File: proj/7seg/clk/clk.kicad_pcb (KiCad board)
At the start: 2 copper layers, 50 x 15 mm, 27 parts, among them J1 Conn_01x02_Pin, J2 USB_A, J3 USB_C_Receptacle_PowerOnly_6P, SW1 SW_Push, SW2 SW_Push, U1 LTC-4627JG, U2 74HC595, U3 74HC595, U4 ATtiny402-SS

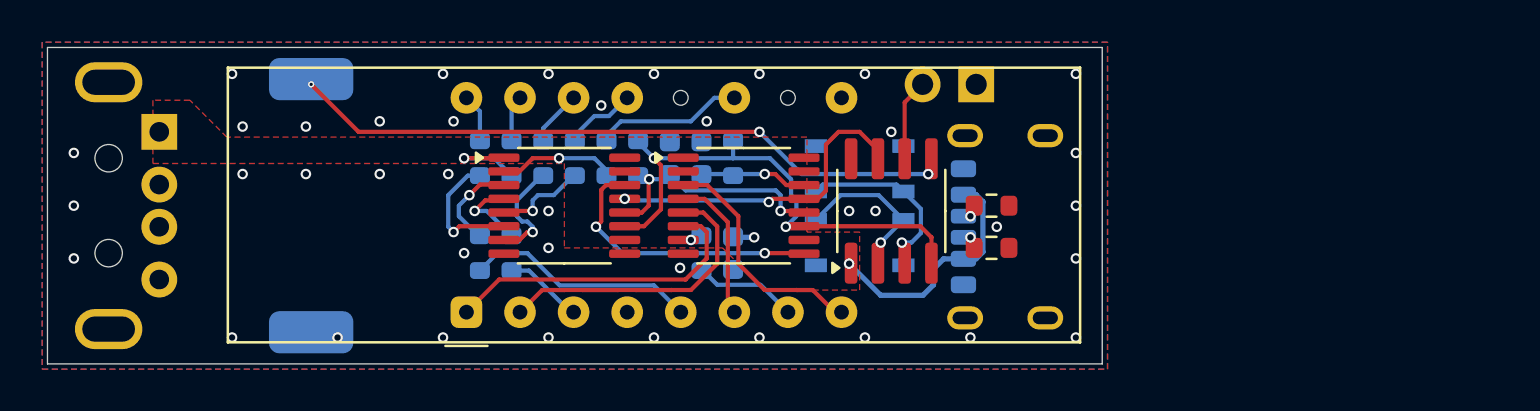
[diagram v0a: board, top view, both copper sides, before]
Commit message: -
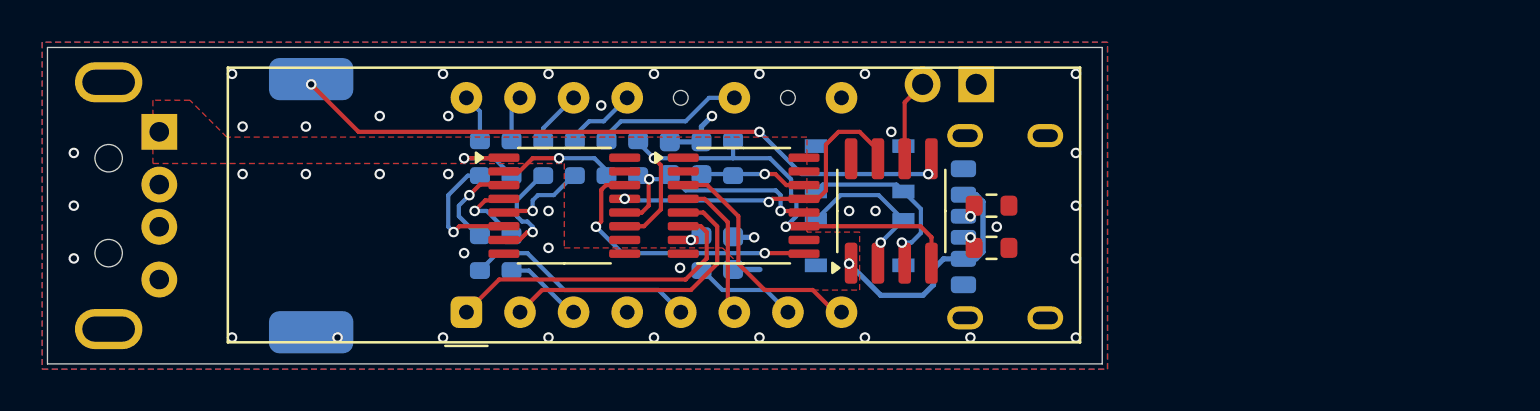
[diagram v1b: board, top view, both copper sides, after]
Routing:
- net GND: track 0.00 -> 4.21 mm
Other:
- board text added: "AVR CLK"
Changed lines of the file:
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@@
 		(layer "Edge.Cuts")
+	)
+	(gr_text "AVR CLK"
+		(at 78.75 102.25 90)
+		(layer "F.Mask")
+		(effects
+			(font
+				(size 1 1)
+				(thickness 0.2)
+				(bold yes)
+			)
+		)
 	)
 	(gr_text "C"
@@
 	)
 	(via
-		(at 90.5 96)
+		(at 90.25 95.75)
 		(size 0.5)
 		(drill 0.3)
@@
 	)
 	(via
-		(at 87 96)
+		(at 87 95.75)
 		(size 0.5)
 		(drill 0.3)
@@
 	)
 	(via
-		(at 102.5 96)
+		(at 102.75 95.75)
 		(size 0.5)
 		(drill 0.3)
@@
 		(layers "F.Cu" "B.Cu")
 		(free yes)
+		(net 2)
+	)
+	(segment
+		(start 100.75 96.975)
+		(end 102.25 96.975)
+		(width 0.25)
+		(layer "B.Cu")
+		(net 2)
+	)
+	(segment
+		(start 102.25 96.975)
+		(end 102.25 96.25)
+		(width 0.25)
+		(layer "B.Cu")
+		(net 2)
+	)
+	(segment
+		(start 103.75 103.025)
+		(end 105.025 103.025)
+		(width 0.25)
+		(layer "B.Cu")
+		(net 2)
+	)
+	(segment
+		(start 102.25 96.25)
+		(end 102.75 95.75)
+		(width 0.25)
+		(layer "B.Cu")
 		(net 2)
 	)
@@
 	(via
 		(at 83.75 94.25)
-		(size 0.3)
-		(drill 0.15)
+		(size 0.5)
+		(drill 0.3)
 		(layers "F.Cu" "B.Cu")
 		(net 9)
@@
 	)
 	(segment
-		(start 97.8675 95.75)
-		(end 98.73 94.8875)
-		(width 0.2)
-		(layer "B.Cu")
-		(net 14)
-	)
-	(segment
-		(start 96.25 96.675)
-		(end 97.175 95.75)
-		(width 0.2)
-		(layer "B.Cu")
-		(net 14)
-	)
-	(segment
 		(start 96.25 96.925)
 		(end 96.25 96.675)
@@
 	)
 	(segment
-		(start 97.175 95.75)
-		(end 97.8675 95.75)
+		(start 96.925 96)
+		(end 97.6175 96)
+		(width 0.2)
+		(layer "B.Cu")
+		(net 14)
+	)
+	(segment
+		(start 97.6175 96)
+		(end 98.73 94.8875)
+		(width 0.2)
+		(layer "B.Cu")
+		(net 14)
+	)
+	(segment
+		(start 96.25 96.675)
+		(end 96.925 96)
 		(width 0.2)
 		(layer "B.Cu")
@@
 	)
 	(segment
-		(start 91.75 103.075)
+		(start 100.219 103.9965)
+		(end 95.7465 103.9965)
+		(width 0.2)
+		(layer "B.Cu")
+		(net 18)
+	)
+	(segment
+		(start 101.27 105.0475)
+		(end 100.219 103.9965)
+		(width 0.2)
+		(layer "B.Cu")
+		(net 18)
+	)
+	(segment
+		(start 94 102.25)
 		(end 92.575 102.25)
 		(width 0.2)
@@
 	)
 	(segment
-		(start 95.526 103.776)
-		(end 99.9985 103.776)
+		(start 95.7465 103.9965)
+		(end 94 102.25)
 		(width 0.2)
 		(layer "B.Cu")
@@
 	)
 	(segment
-		(start 99.9985 103.776)
-		(end 101.27 105.0475)
-		(width 0.2)
-		(layer "B.Cu")
-		(net 18)
-	)
-	(segment
-		(start 94 102.25)
-		(end 95.526 103.776)
-		(width 0.2)
-		(layer "B.Cu")
-		(net 18)
-	)
-	(segment
 		(start 92.575 102.25)
-		(end 94 102.25)
+		(end 91.75 103.075)
 		(width 0.2)
 		(layer "B.Cu")
@@
 	)
 	(segment
+		(start 102.6125 94.8875)
+		(end 101.5 96)
+		(width 0.2)
+		(layer "B.Cu")
+		(net 20)
+	)
+	(segment
 		(start 103.81 94.8875)
-		(end 102.8625 94.8875)
+		(end 102.6125 94.8875)
 		(width 0.2)
 		(layer "B.Cu")
@@
 	)
 	(segment
-		(start 102.8625 94.8875)
-		(end 101.75 96)
-		(width 0.2)
-		(layer "B.Cu")
-		(net 20)
-	)
-	(segment
-		(start 101.75 96)
-		(end 98.429251 96)
+		(start 98.429251 96)
+		(end 97.75 96.679251)
 		(width 0.2)
 		(layer "B.Cu")
@@
 	)
 	(segment
-		(start 98.429251 96)
-		(end 97.75 96.679251)
+		(start 101.5 96)
+		(end 98.429251 96)
 		(width 0.2)
 		(layer "B.Cu")
@@
 	)
 	(segment
-		(start 105.0525 103.75)
-		(end 106.35 105.0475)
-		(width 0.2)
-		(layer "B.Cu")
-		(net 24)
-	)
-	(segment
-		(start 102.325 103.075)
-		(end 103 103.75)
-		(width 0.2)
-		(layer "B.Cu")
-		(net 24)
-	)
-	(segment
-		(start 103 103.75)
-		(end 105.0525 103.75)
-		(width 0.2)
-		(layer "B.Cu")
-		(net 24)
-	)
-	(segment
 		(start 102.25 103.075)
 		(end 102.325 103.075)
@@
 		(net 24)
 	)
+	(segment
+		(start 102.325 103.075)
+		(end 103.2465 103.9965)
+		(width 0.2)
+		(layer "B.Cu")
+		(net 24)
+	)
+	(segment
+		(start 103.2465 103.9965)
+		(end 105.299 103.9965)
+		(width 0.2)
+		(layer "B.Cu")
+		(net 24)
+	)
+	(segment
+		(start 105.299 103.9965)
+		(end 106.35 105.0475)
+		(width 0.2)
+		(layer "B.Cu")
+		(net 24)
+	)
 	(via
 		(at 101.75 101.625)
@@
 	)
 	(segment
-		(start 106.788839 104)
-		(end 107.53013 104)
-		(width 0.2)
-		(layer "F.Cu")
-		(net 32)
-	)
-	(segment
 		(start 102.525 99.025)
 		(end 104 100.5)
@@
 	)
 	(segment
+		(start 101.3875 99.025)
+		(end 102.525 99.025)
+		(width 0.2)
+		(layer "F.Cu")
+		(net 32)
+	)
+	(segment
+		(start 108.57763 105.0475)
+		(end 108.89 105.0475)
+		(width 0.2)
+		(layer "F.Cu")
+		(net 32)
+	)
+	(segment
 		(start 104 102.75)
 		(end 105.2465 103.9965)
@@
 	)
 	(segment
-		(start 106.785339 103.9965)
-		(end 106.788839 104)
-		(width 0.2)
-		(layer "F.Cu")
-		(net 32)
-	)
-	(segment
-		(start 105.2465 103.9965)
-		(end 106.785339 103.9965)
-		(width 0.2)
-		(layer "F.Cu")
-		(net 32)
-	)
-	(segment
-		(start 108.57763 105.0475)
-		(end 108.89 105.0475)
-		(width 0.2)
-		(layer "F.Cu")
-		(net 32)
-	)
-	(segment
-		(start 101.3875 99.025)
-		(end 102.525 99.025)
-		(width 0.2)
-		(layer "F.Cu")
-		(net 32)
-	)
-	(segment
-		(start 107.53013 104)
+		(start 107.52663 103.9965)
 		(end 108.57763 105.0475)
 		(width 0.2)
@@
 	)
 	(segment
+		(start 105.2465 103.9965)
+		(end 107.52663 103.9965)
+		(width 0.2)
+		(layer "F.Cu")
+		(net 32)
+	)
+	(segment
 		(start 102.225 100.975)
 		(end 102.5 101.25)
@@
 	)
 	(segment
-		(start 94.6975 104)
-		(end 93.65 105.0475)
+		(start 101.3875 100.325)
+		(end 102.341426 100.325)
+		(width 0.2)
+		(layer "F.Cu")
+		(net 34)
+	)
+	(segment
+		(start 101.7535 103.9965)
+		(end 94.701 103.9965)
+		(width 0.2)
+		(layer "F.Cu")
+		(net 34)
+	)
+	(segment
+		(start 102.341426 100.325)
+		(end 103 100.983574)
 		(width 0.2)
 		(layer "F.Cu")
@@
 	)
 	(segment
-		(start 95.754661 103.9965)
-		(end 95.751161 104)
-		(width 0.2)
-		(layer "F.Cu")
-		(net 34)
-	)
-	(segment
-		(start 98.291161 104)
-		(end 96.628839 104)
-		(width 0.2)
-		(layer "F.Cu")
-		(net 34)
-	)
-	(segment
-		(start 99.168839 104)
-		(end 99.165339 103.9965)
-		(width 0.2)
-		(layer "F.Cu")
-		(net 34)
-	)
-	(segment
-		(start 95.751161 104)
-		(end 94.6975 104)
-		(width 0.2)
-		(layer "F.Cu")
-		(net 34)
-	)
-	(segment
-		(start 102.341426 100.325)
-		(end 103 100.983574)
-		(width 0.2)
-		(layer "F.Cu")
-		(net 34)
-	)
-	(segment
-		(start 96.625339 103.9965)
-		(end 95.754661 103.9965)
-		(width 0.2)
-		(layer "F.Cu")
-		(net 34)
-	)
-	(segment
-		(start 99.165339 103.9965)
-		(end 98.294661 103.9965)
-		(width 0.2)
-		(layer "F.Cu")
-		(net 34)
-	)
-	(segment
-		(start 98.294661 103.9965)
-		(end 98.291161 104)
-		(width 0.2)
-		(layer "F.Cu")
-		(net 34)
-	)
-	(segment
-		(start 100.831161 104)
-		(end 99.168839 104)
-		(width 0.2)
-		(layer "F.Cu")
-		(net 34)
-	)
-	(segment
-		(start 100.834661 103.9965)
-		(end 100.831161 104)
-		(width 0.2)
-		(layer "F.Cu")
-		(net 34)
-	)
-	(segment
-		(start 101.7535 103.9965)
-		(end 100.834661 103.9965)
+		(start 94.701 103.9965)
+		(end 93.65 105.0475)
 		(width 0.2)
 		(layer "F.Cu")
@@
 		(width 0.2)
 		(layer "F.Cu")
-		(net 34)
-	)
-	(segment
-		(start 101.3875 100.325)
-		(end 102.341426 100.325)
-		(width 0.2)
-		(layer "F.Cu")
-		(net 34)
-	)
-	(segment
-		(start 96.628839 104)
-		(end 96.625339 103.9965)
-		(width 0.2)
-		(layer "F.Cu")

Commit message: -
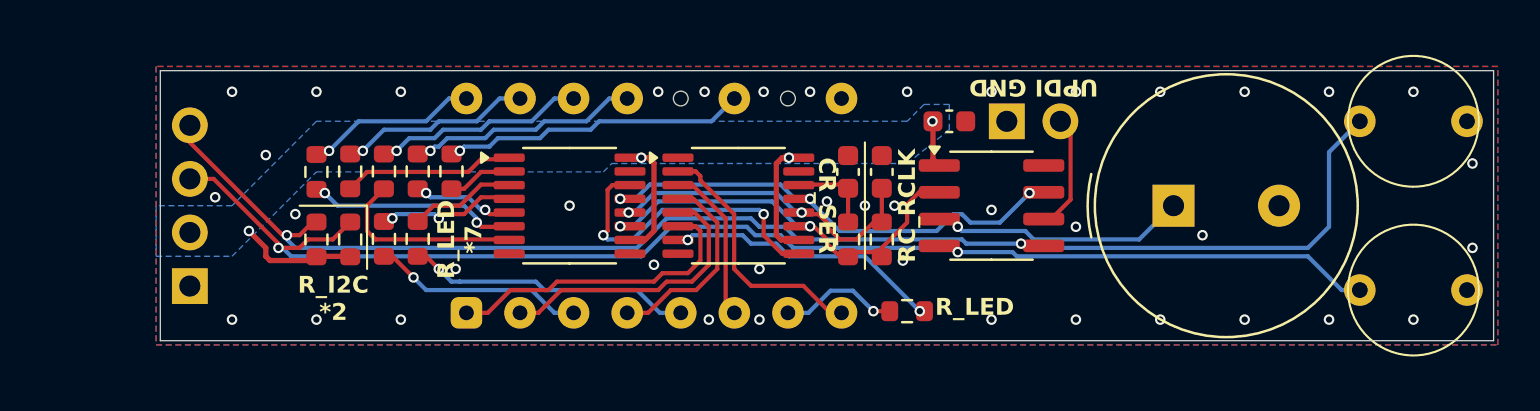
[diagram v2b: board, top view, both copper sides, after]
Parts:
- removed J3: USB_C_Receptacle_PowerOnly_6P, Connector_USB:USB_C_Receptacle_GCT_USB4125-xx-x_6P_TopMnt_Horizontal
- removed LS1: Speaker, Library:PKLCS1212E4001-R1
- added BZ1: Buzzer, Buzzer_Beeper:Buzzer_TDK_PS1240P02BT_D12.2mm_H6.5mm, F.Cu at (124.6, 100.0)
- ?: moved to B.Cu
- C1: value C_Small -> C_RCLK; moved to F.Cu
- C2: value C_Small -> C_SER; moved to F.Cu
- C3, R1, R2, R3, R4, R5, R6, R7, R8: moved to F.Cu
- J2: value USB_A -> Conn_01x04_Pin; footprint Library:USB_A_PLUG_USB-4AM103AS -> Connector_PinHeader_2.54mm:PinHeader_1x04_P2.54mm_Vertical; moved to B.Cu
- R10: value R_Small -> R_SER; moved to F.Cu
- R11, R12: value 5k1 -> R_I2C
- R9: value R_Small -> R_RCLK; moved to F.Cu
- SW1, SW2: footprint Library:alps-skrp -> Library:alps-skrg; moved to F.Cu
- moved ? 52.0 mm to (136.0, 100.0), turned to -90 degrees
- moved G*** 43.4 mm to (127.0, 97.0), turned to -90 degrees
- moved R12 32.0 mm to (84.0, 101.6), turned to 90 degrees
- moved R11 30.4 mm to (85.6, 101.6), turned to 90 degrees
- moved SW1 26.3 mm to (136.0, 104.0)
- moved SW2 26.3 mm to (136.0, 96.0), turned to 0 degrees
- moved R9 12.2 mm to (110.8, 101.6), turned to 90 degrees
- moved C3 12.0 mm to (114.0, 96.0), turned to 0 degrees
- moved R8 10.1 mm to (112.0, 105.0), turned to 180 degrees
- moved C1 10.1 mm to (110.8, 98.4)
- moved R2 7.78 mm to (84.0, 98.4)
- moved J2 7.75 mm to (78.0, 103.8), turned to 0 degrees
- moved R7 7.68 mm to (85.6, 98.4)
- moved R1 7.58 mm to (87.2, 98.4)
- moved R3 7.48 mm to (88.8, 98.4)
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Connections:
- J2 pad 1: VCC -> GND
- J2 pad 2: unconnected-(J2-D--Pad2) -> VCC
- J2 pad 3: unconnected-(J2-D+-Pad3) -> PA1
- J2 pad 4: GND -> PA2
- R1 pad 1: /_SEG0 -> /_SEG1
- R1 pad 2: SEG0 -> SEG1
- R11 pad 1: Net-(J3-CC1) -> VCC
- R11 pad 2: GND -> PA1
- R12 pad 1: Net-(J3-CC2) -> VCC
- R12 pad 2: GND -> PA2
- R2 pad 1: /_SEG1 -> /_SEG2
- R2 pad 2: SEG1 -> SEG2
- R3 pad 1: /_SEG2 -> /_SEG3
- R3 pad 2: SEG2 -> SEG3
- R4 pad 1: /_SEG3 -> /_SEG4
- R4 pad 2: SEG3 -> SEG4
- R5 pad 1: /_SEG4 -> /_SEG5
- R5 pad 2: SEG4 -> SEG5
- R6 pad 1: /_SEG5 -> /_SEG6
- R6 pad 2: SEG5 -> SEG6
- R7 pad 1: /_SEG6 -> /_SEG7
- R7 pad 2: SEG6 -> SEG7
- R8 pad 1: /_SEG7 -> /_SEG8
- R8 pad 2: SEG7 -> SEG8
- SW1 pad 1: BTN0 -> PA1
- SW2 pad 1: BTN1 -> PA2
- U1 pad 1: SEGC0 -> SEGC1
- U1 pad 11: SEG5 -> SEG6
- U1 pad 13: SEG2 -> SEG3
- U1 pad 14: SEG0 -> SEG1
- U1 pad 15: SEG6 -> SEG7
- U1 pad 16: SEG1 -> SEG2
- U1 pad 2: SEGC1 -> SEGC2
- U1 pad 3: SEG3 -> SEG4
- U1 pad 4: SEGC4 -> SEGC:
- U1 pad 5: SEG4 -> SEG5
- U1 pad 6: SEGC2 -> SEGC3
- U1 pad 7: SEG7 -> SEG8
- U1 pad 8: SEGC3 -> SEGC4
- U2 pad 1: /_SEG6 -> /_SEG7
- U2 pad 2: /_SEG5 -> /_SEG6
- U2 pad 3: /_SEG4 -> /_SEG5
- U2 pad 4: /_SEG3 -> /_SEG4
- U2 pad 5: /_SEG2 -> /_SEG3
- U2 pad 6: /_SEG1 -> /_SEG2
- U2 pad 7: /_SEG0 -> /_SEG1
- U3 pad 2: unconnected-(U3-QC-Pad2) -> SEGC4
- U3 pad 4: SEGC2 -> SEGC:
- U3 pad 5: SEGC1 -> SEGC2
- U3 pad 6: SEGC0 -> SEGC1
- U3 pad 7: /_SEG7 -> /_SEG8
- U4 pad 2: BTN0 -> SRCLK
- U4 pad 3: BTN1 -> SPK
- U4 pad 4: SRCLK -> PA1
- U4 pad 5: SPK -> PA2
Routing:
- net PA2: track 0.00 -> 65.8 mm, vias 0 -> 2
- net PA1: track 0.00 -> 63.9 mm, vias 0 -> 2
- net SPK: track 31.0 -> 11.1 mm, vias 3 -> 1
- net SEGC0: track 14.9 -> 0.00 mm
- net /_SEG8: track 0.00 -> 13.3 mm, vias 0 -> 2
- net SEG6: track 2.20 -> 14.5 mm, vias 0 -> 1
- net SEGC4: track 0.00 -> 12.2 mm
- net SEGC:: track 0.00 -> 9.66 mm
- net /_SEG7: track 0.00 -> 8.15 mm, vias 1 -> 0
- net OE#: track 15.5 -> 23.4 mm, vias 2 -> 3
- net BTN1: track 7.82 -> 0.00 mm, vias 1 -> 0
- net SEG1: track 2.30 -> 10.1 mm, vias 0 -> 1
- net SEG3: track 3.76 -> 11.0 mm, vias 0 -> 1
- net BTN0: track 6.64 -> 0.00 mm, vias 1 -> 0
- net SEG5: track 7.05 -> 13.6 mm, vias 0 -> 1
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- added copper zone on B.Cu, net VCC
- removed copper zone on F.Cu, net VCC
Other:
- board size 50 x 15 mm -> 63.2 x 12.8 mm
- board text added: "CR_SER"
- board text added: "RC_RCLK"
- board text added: "R_I2C *2"
- board text added: "R_LED"
- board text added: "R_LED *7"
- board text added: "UPDI GND"
- board text removed: "AVR CLK"
- board text removed: "C"
- board text removed: "PA2"
- board text removed: "PA6"
- board text removed: "PA7"
- board text removed: "RCLK"
- board text removed: "RC|CR"
- board text removed: "R_LED x8"
- board text removed: "SER"
- board text removed: "UPDI"
